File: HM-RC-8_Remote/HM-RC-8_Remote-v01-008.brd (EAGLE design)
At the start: 70 x 22 mm, 18 parts, among them M2 ARDUINO-PRO-MINI-3.3V#NP

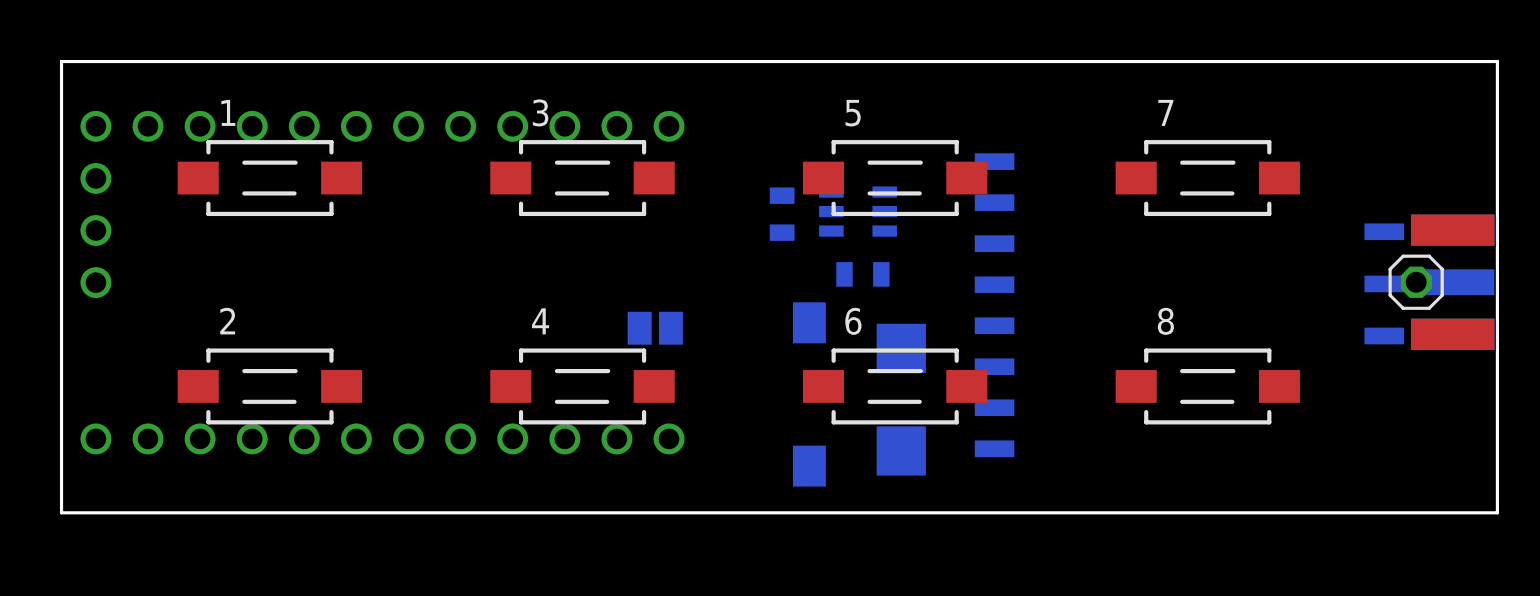
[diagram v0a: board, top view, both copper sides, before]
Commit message: Remote
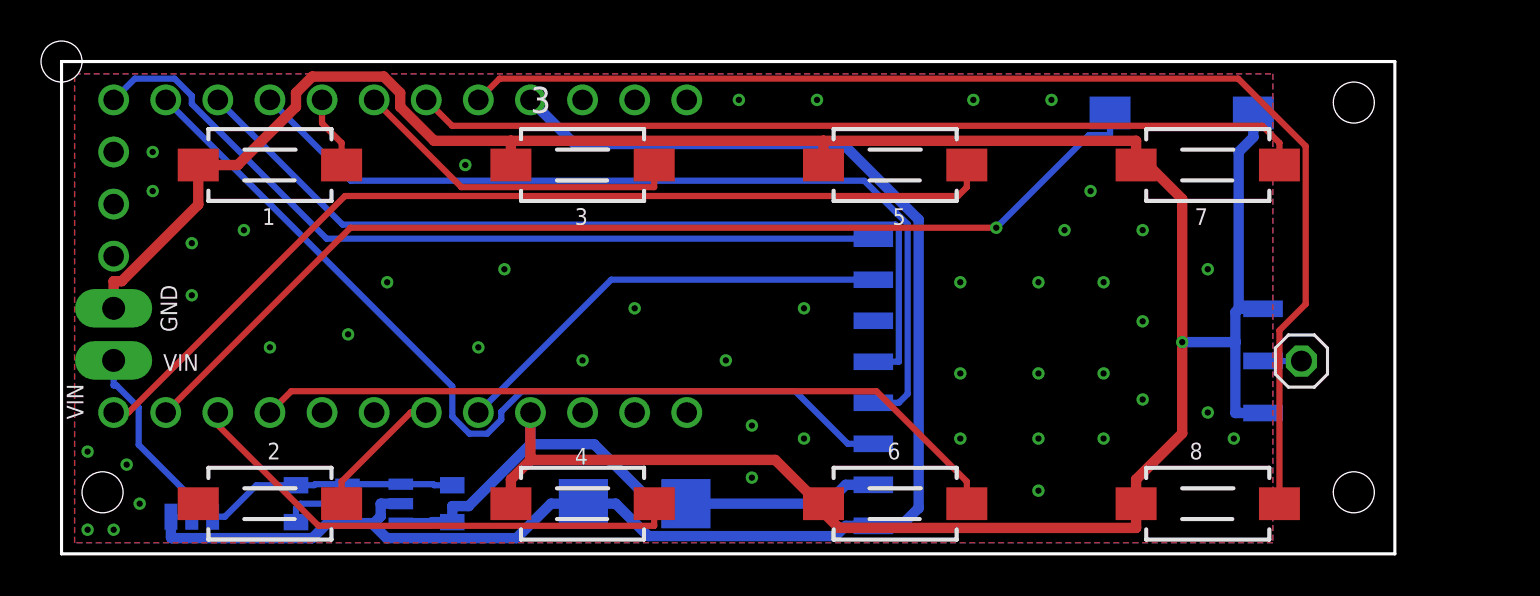
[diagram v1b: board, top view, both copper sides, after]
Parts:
- removed RAW: (no value), jumper:SJ
- removed X5: (no value), adafruit:SMA_EDGELAUNCH
- added J1: (no value), SparkFun-Connectors:1X02_LONGPADS
- added JP1: JUMPER-SMT_3_1-NC_TRACE_SILK, SparkFun-Jumpers:SMT-JUMPER_3_1-NC_TRACE_SILK
- moved L1 27.6 mm to (11.4, 4.45)
- moved STEPUP 27.6 mm to (15.2, 4.45)
- moved C5 22.9 mm to (19.1, 4.45), turned to 270 degrees
- moved ICLUSION 22.8 mm to (54.6, 23.5), turned to 0 degrees
- moved C3 14.0 mm to (27.9, 4.45), turned to 180 degrees
- moved CC0 7.00 mm to (39.6, 17.4)
- moved ANT 6.79 mm to (60.4, 11.4)
- moved 2 5.71 mm to (10.2, 4.45)
- moved 4 5.71 mm to (25.4, 4.45)
- moved 6 5.71 mm to (40.6, 4.45)
- moved 8 5.71 mm to (55.9, 4.45)
- moved M2 1.55 mm to (17.8, 16.5)
- moved 1 0.63 mm to (10.2, 21.0)
- moved 3 0.63 mm to (25.4, 21.0)
- moved 5 0.63 mm to (40.6, 21.0)
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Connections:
- removed net N$10: 8.2
- removed net N$6: 4.2
- removed net N$7: 5.2
- removed net N$8: 6.2
- removed net N$9: 7.2
- removed net UREG: RAW.2
- new net N$4: J1.1, JP1.2
- net 16-A2: now also 7.2
- net 17-A3: now also 8.2
- net ANT0: no longer X5.P
- net D6: now also 6.2
- net D7: now also 4.2
- net D9: now also 5.2
- net GND: now also J1.2; no longer X5.GND@1, X5.GND@2, X5.GND@3, X5.GND@4
- net RAW: no longer RAW.1
- net VCC: now also JP1.3
- net VIN: now also JP1.1
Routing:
- net GND: track 0.00 -> 166.6 mm, vias 0 -> 46
- net VCC: track 0.00 -> 77.5 mm
- net 17-A3: track 0.00 -> 60.1 mm
- net D8: track 0.00 -> 52.7 mm, vias 0 -> 1
- net D9: track 0.00 -> 47.2 mm
- net MOSI: track 0.00 -> 44.2 mm
- net SCK: track 0.00 -> 43.7 mm
- net MISO: track 0.00 -> 43.6 mm
- net 16-A2: track 0.00 -> 43.5 mm
- net CSN: track 0.00 -> 40.9 mm
- net D6: track 0.00 -> 37.3 mm
- net D7: track 0.00 -> 25.0 mm
- net IRQ: track 0.00 -> 21.9 mm
- net 15-A1: track 0.00 -> 16.5 mm
- net VIN: track 0.00 -> 12.4 mm
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- added copper zone on layer 1, net GND
- added copper zone on layer 16, net GND
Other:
- board size 70 x 22 mm -> 65 x 24 mm
- board text added: "1"
- board text added: "2"
- board text added: "3"
- board text added: "4"
- board text added: "5"
- board text added: "6"
- board text added: "7"
- board text added: "8"
- board text added: "C3"
- board text added: "C5"
- board text added: "GND"
- board text added: "L1"
- board text added: "Pairing"
- board text added: "StepUp"
- board text added: "TLV61224"
- board text added: "VIN"
